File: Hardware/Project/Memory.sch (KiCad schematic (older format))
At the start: 3 parts, among them U10 28C256, U12 28C256, U9 7400

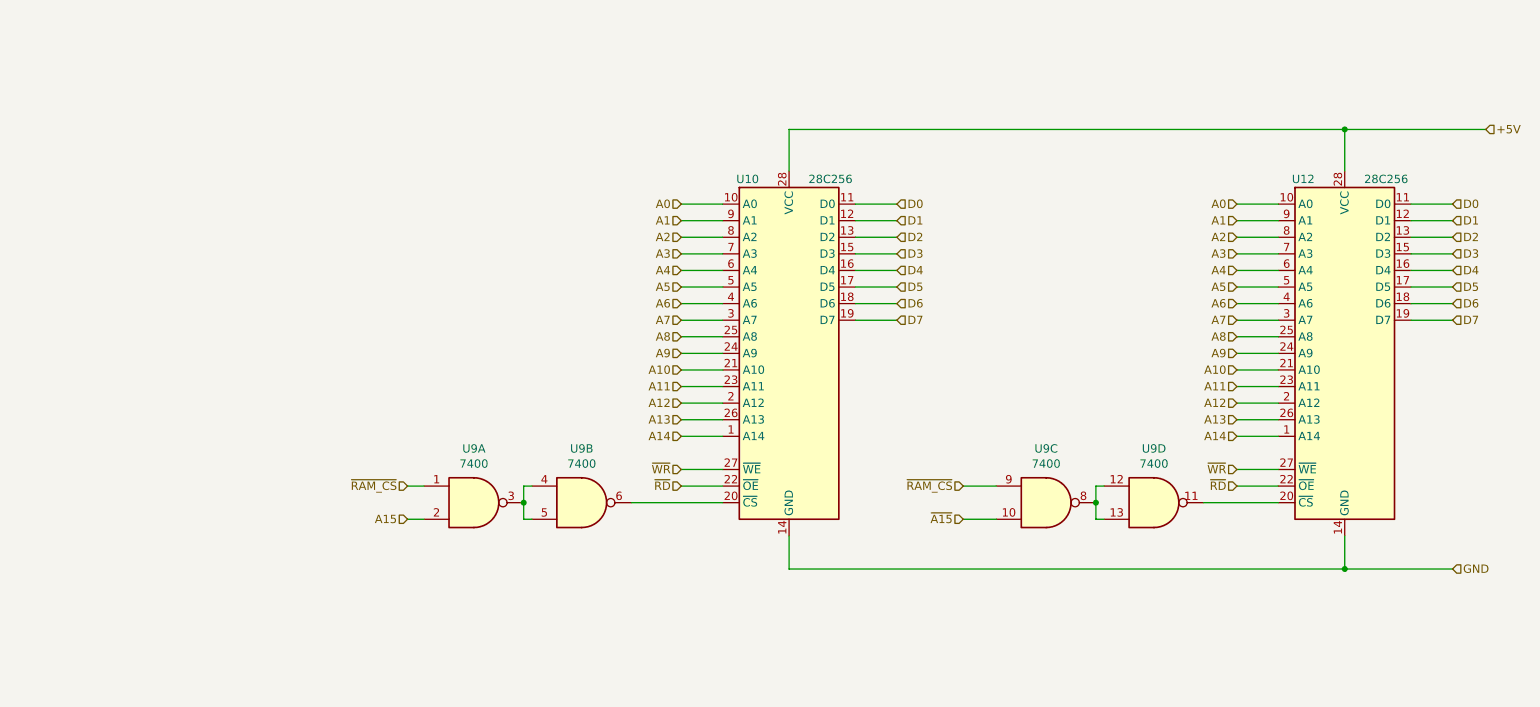
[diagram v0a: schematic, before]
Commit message: 1
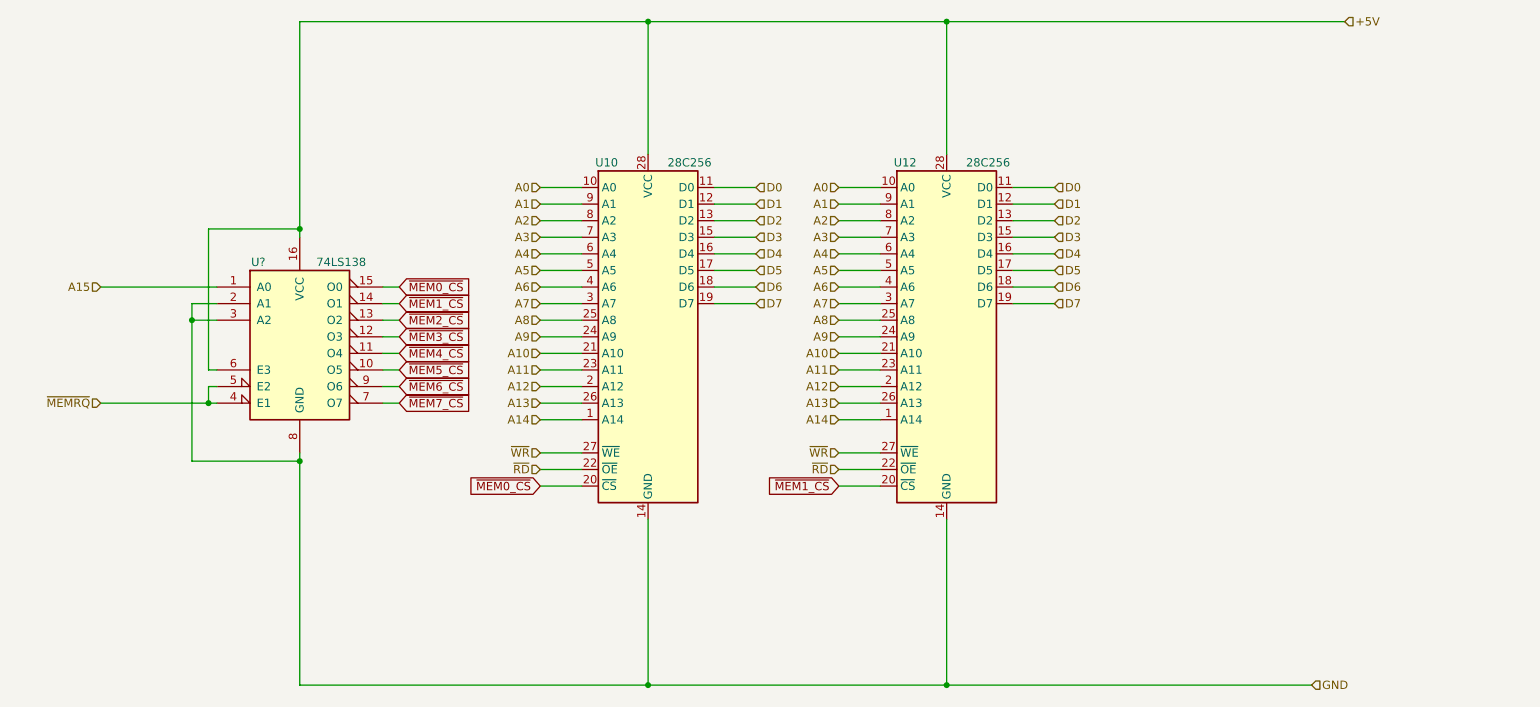
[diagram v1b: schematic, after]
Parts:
- removed U9: 7400, symbol 74xx:7400
- added U?: 74LS138, symbol 74xx:74LS138
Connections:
- net +5V: now also U?.16 (VCC), U?.6 (E3)
- net A15: now also U?.1 (A0)
- net GND: now also U?.2 (A1), U?.3 (A2), U?.8 (GND)
- net ~MEM0_CS: now reaches U10.20 (~CS)
- net ~MEM0_CS: now also U?.15 (O0)
- net ~MEM1_CS: now reaches U12.20 (~CS)
- net ~MEM1_CS: now also U?.14 (O1)
- new net ~MEM2_CS: U?.13 (O2)
- new net ~MEM3_CS: U?.12 (O3)
- new net ~MEM4_CS: U?.11 (O4)
- new net ~MEM5_CS: U?.10 (O5)
- new net ~MEM6_CS: U?.9 (O6)
- new net ~MEM7_CS: U?.7 (O7)
- new net ~MEMRQ: U?.4 (E1), U?.5 (E2)
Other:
- moved on the sheet: U10, U12
